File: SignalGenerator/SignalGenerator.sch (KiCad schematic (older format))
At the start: 31 parts

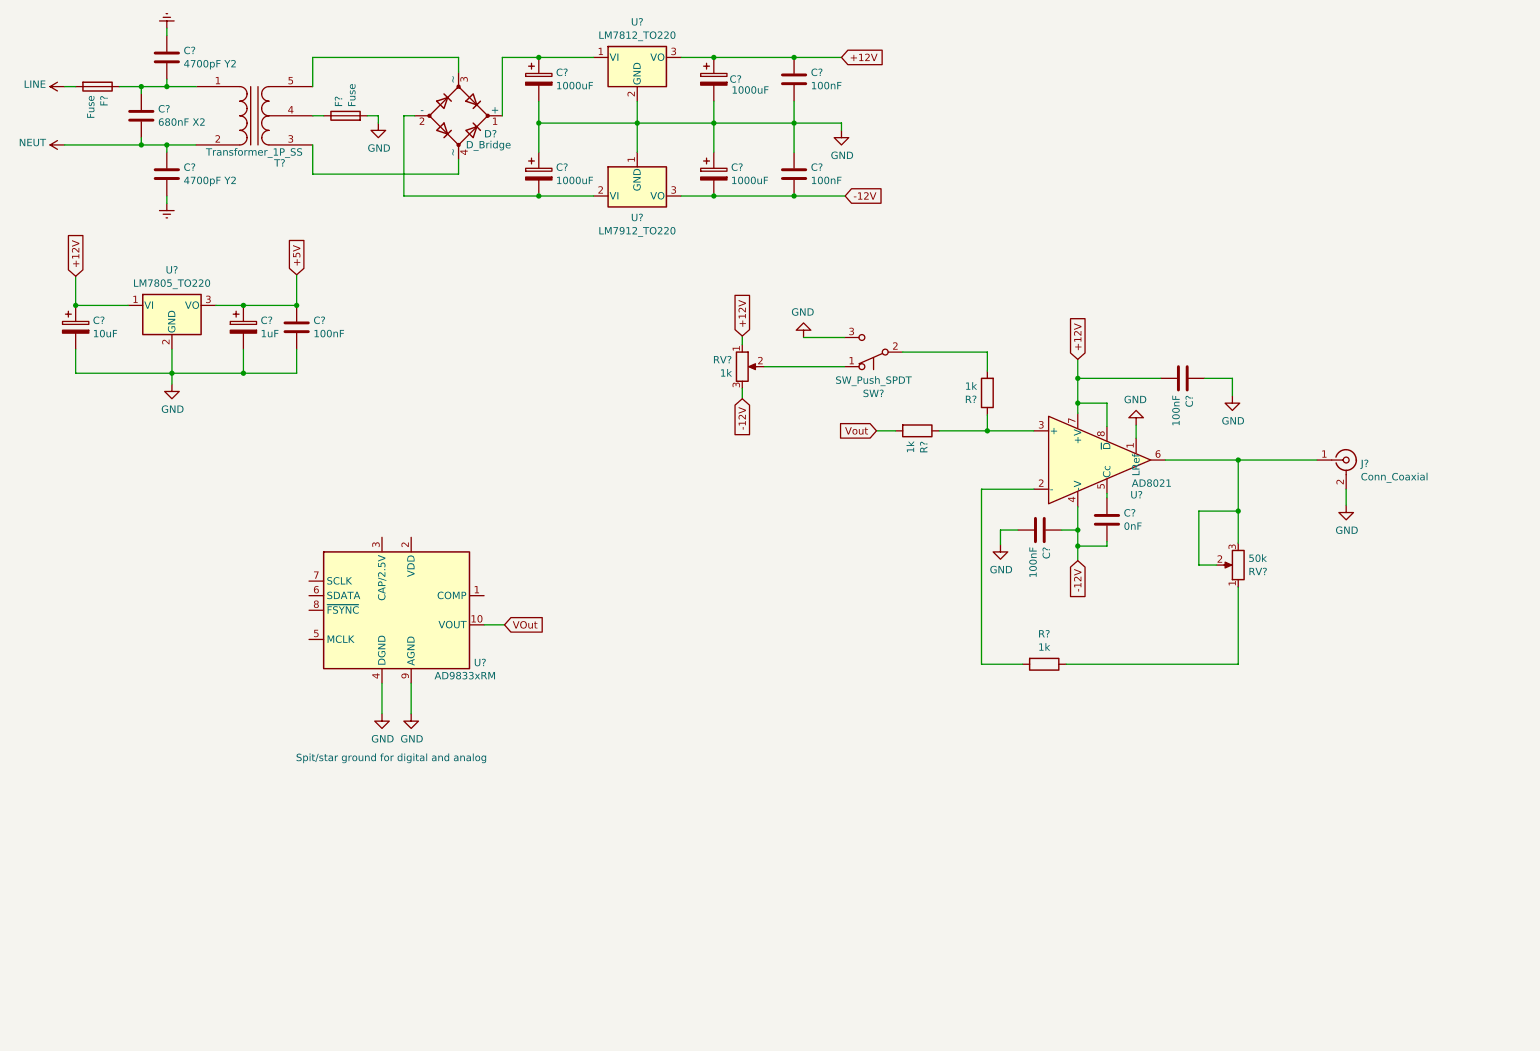
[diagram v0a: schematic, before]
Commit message: Made alot off changes. schematics is much closer to done
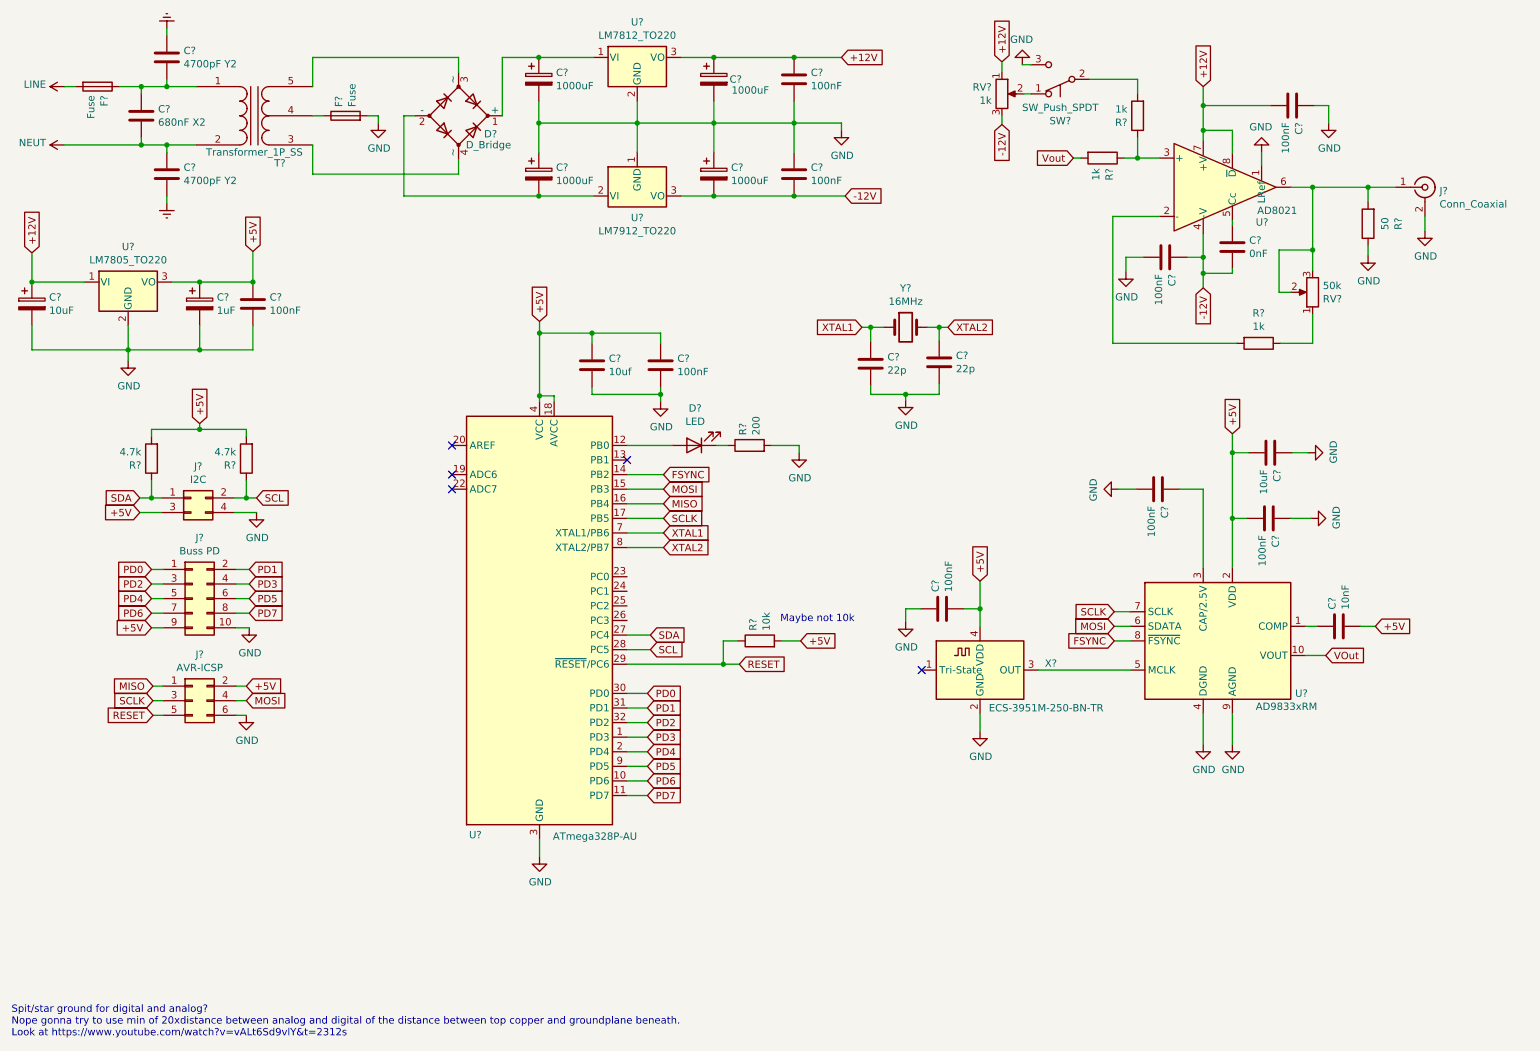
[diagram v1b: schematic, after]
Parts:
- added C? (x4): 100nF, symbol Device:C
- added C?: 10uF, symbol Device:C
- added C?: 10uf, symbol Device:C
- added C? (x2): 22p, symbol Device:C
- added C?: 10nF, symbol Device:C
- added D?: LED, symbol Device:LED
- added J?: AVR-ICSP, symbol Connector_Generic:Conn_02x03_Odd_Even
- added J?: Buss PD, symbol Connector_Generic:Conn_02x05_Odd_Even
- added J?: I2C, symbol Connector_Generic:Conn_02x02_Odd_Even
- added R?: 50, symbol Device:R
- added R?: 10k, symbol Device:R
- added R?: 200, symbol Device:R
- added R? (x2): 4.7k, symbol Device:R
- added U?: ATmega328P-AU, Package_QFP:TQFP-32_7x7mm_P0.8mm, symbol MCU_Microchip_ATmega:ATmega328P-AU
- added X?: ECS-3951M-250-BN-TR, SignalGenerator:ECS-3951M-250-BN-TR, symbol Oscillator:ECS-2520MV-xxx-xx
- added Y?: 16MHz, symbol Device:Crystal
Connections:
- net +5V: now also U?.2 (VDD), C?.1, C?.1, C?.2, C?.2, C?.2, C?.2, J?.2 (Pin_2), J?.3 (Pin_3), J?.9 (Pin_9), R?.2, R?.2, R?.2, U?.18 (AVCC), U?.4 (VCC), U?.6 (VCC), X?.4 (VDD)
- net GND: now also C?.1, C?.1, C?.1, C?.2, C?.2, C?.2, C?.2, C?.2, J?.10 (Pin_10), J?.4 (Pin_4), J?.6 (Pin_6), R?.1, R?.2, U?.21 (GND), U?.3 (GND), U?.5 (GND), X?.2 (GND)
- net at U?.1 (COMP): now also C?.1
- net at U?.3 (CAP/2.5V): now also C?.1
- net at U?.5 (MCLK): now also X?.3 (OUT)
- net MOSI: now reaches U?.6 (SDATA)
- net MOSI: now also J?.4 (Pin_4), U?.15 (PB3)
- net SCLK: now reaches U?.7 (SCLK)
- net SCLK: now also J?.3 (Pin_3), U?.17 (PB5)
- net FSYNC: now reaches U?.8 (~FSYNC)
- net FSYNC: now also U?.14 (PB2)
- net at J?.1 (In), RV?.2, RV?.3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: now also R?.2
- new net: D?.2 (A), U?.12 (PB0)
- new net: D?.1 (K), R?.1
- new net MISO: J?.1 (Pin_1), U?.16 (PB4)
- new net PD0: J?.1 (Pin_1), U?.30 (PD0)
- new net PD1: J?.2 (Pin_2), U?.31 (PD1)
- new net PD2: J?.3 (Pin_3), U?.32 (PD2)
- new net PD3: J?.4 (Pin_4), U?.1 (PD3)
- new net PD4: J?.5 (Pin_5), U?.2 (PD4)
- new net PD5: J?.6 (Pin_6), U?.9 (PD5)
- new net PD6: J?.7 (Pin_7), U?.10 (PD6)
- new net PD7: J?.8 (Pin_8), U?.11 (PD7)
- new net RESET: J?.5 (Pin_5), R?.1, U?.29 (~RESET~/PC6)
- new net SCL: J?.2 (Pin_2), R?.1, U?.28 (PC5)
- new net SDA: J?.1 (Pin_1), R?.1, U?.27 (PC4)
- new net XTAL1: C?.1, U?.7 (XTAL1/PB6), Y?.1
- new net XTAL2: C?.1, U?.8 (XTAL2/PB7), Y?.2
- no-connect marks 0 -> 5
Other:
- note added: "Maybe not 10k"
- note added: "Spit/star ground for digital and analog?\nNope gonna try to use min of 20xdistance between analog and digital of the distance between top copper and groundplane beneath.\nLook at https://www.youtube.com/watch?v=vALt6Sd9vlY&t=2312s"
- note removed: "Spit/star ground for digital and analog"
- moved on the sheet: C?, J?, R?, RV?, SW?, U?
